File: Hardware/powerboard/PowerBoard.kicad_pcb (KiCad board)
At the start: 2 copper layers, 67 x 66 mm, 95 parts, among them J1 FPC 0.5mm Bottom Contact, J2 DF12NC(3.0)-20DS-0.5V, U1 TPS65130RGE, U2 ADP5071ACPZ, U3 TPS62175DQC, U4 ADP5071ACPZ, U5 TLV74330, U6 TPS65130RGE

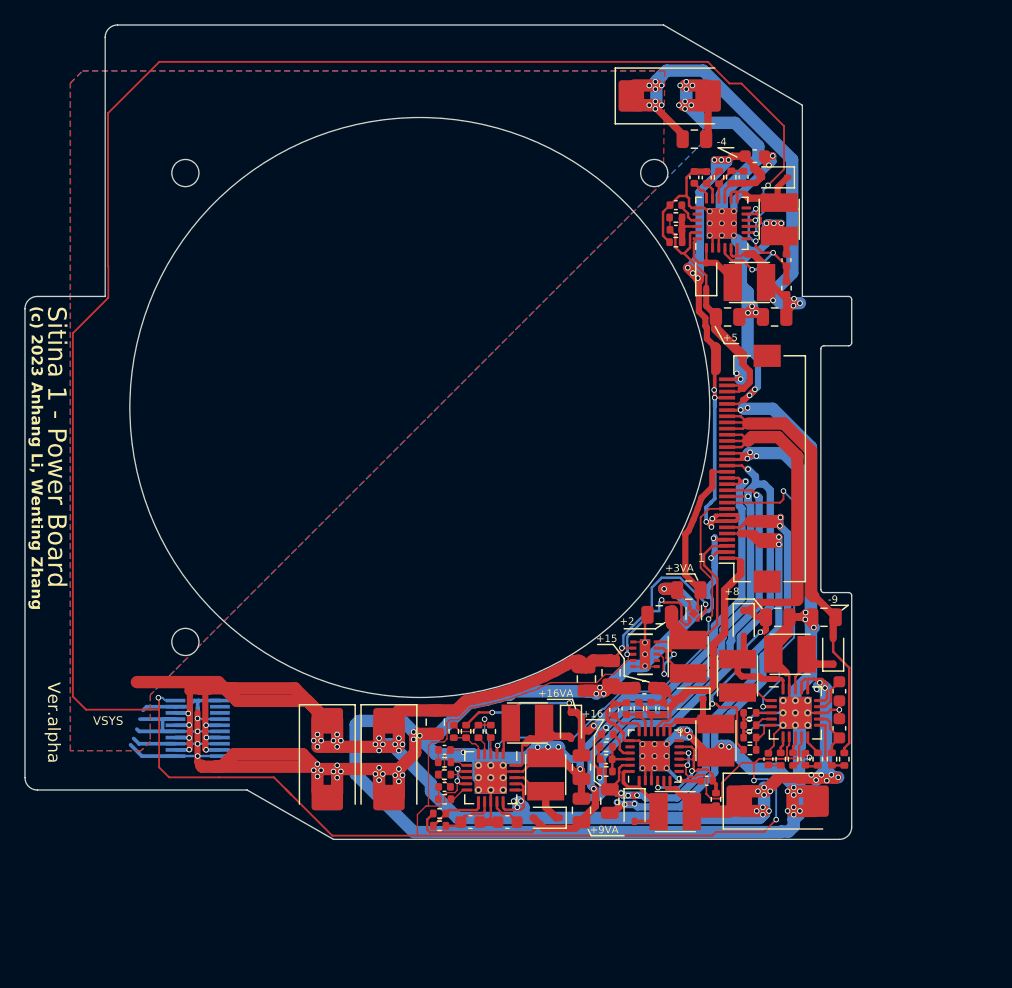
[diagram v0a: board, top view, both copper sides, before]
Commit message: CCD Sensor Board WIP
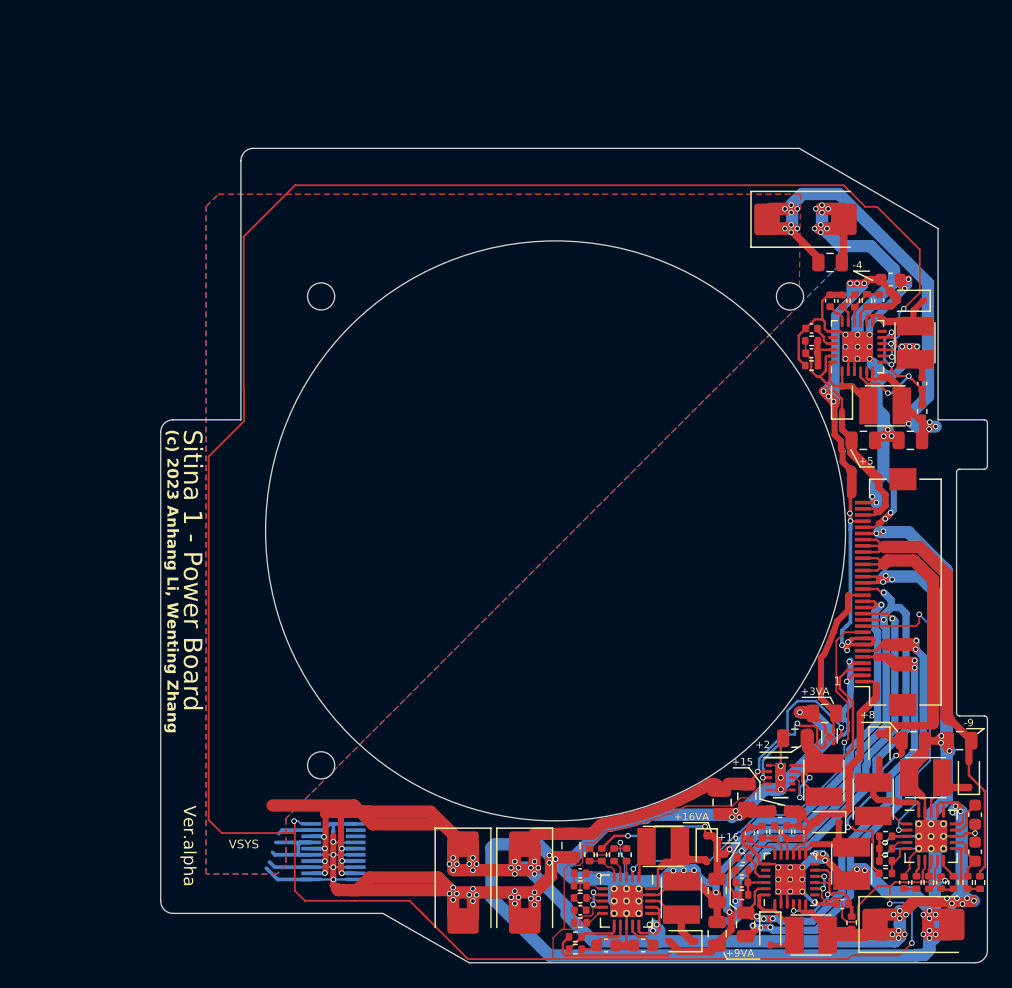
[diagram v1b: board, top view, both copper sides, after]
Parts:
- moved C17 14.9 mm to (184.4, 131.8)
- moved C18 14.9 mm to (186.8, 129.8)
- moved C1 14.9 mm to (187.2, 93.2)
- moved C10 14.9 mm to (178.5, 137.0)
- moved C11 14.9 mm to (199.0, 138.0)
- moved C12 14.9 mm to (193.2, 143.5)
- moved C13 14.9 mm to (196.2, 143.5)
- moved C14 14.9 mm to (199.0, 141.0)
- moved C15 14.9 mm to (197.8, 132.0)
- moved C16 14.9 mm to (194.0, 132.0)
- moved C19 14.9 mm to (180.5, 136.5)
- moved C2 14.9 mm to (194.7, 103.1)
- moved C20 14.9 mm to (166.2, 140.5)
- moved C22 14.9 mm to (188.2, 145.2)
- moved C23 14.9 mm to (181.8, 139.4)
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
